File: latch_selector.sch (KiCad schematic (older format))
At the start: 15 parts, among them SW1 SW_Coded_Octal-8, U1 74HCT138, U2 74HCT151, U6 74HCT32

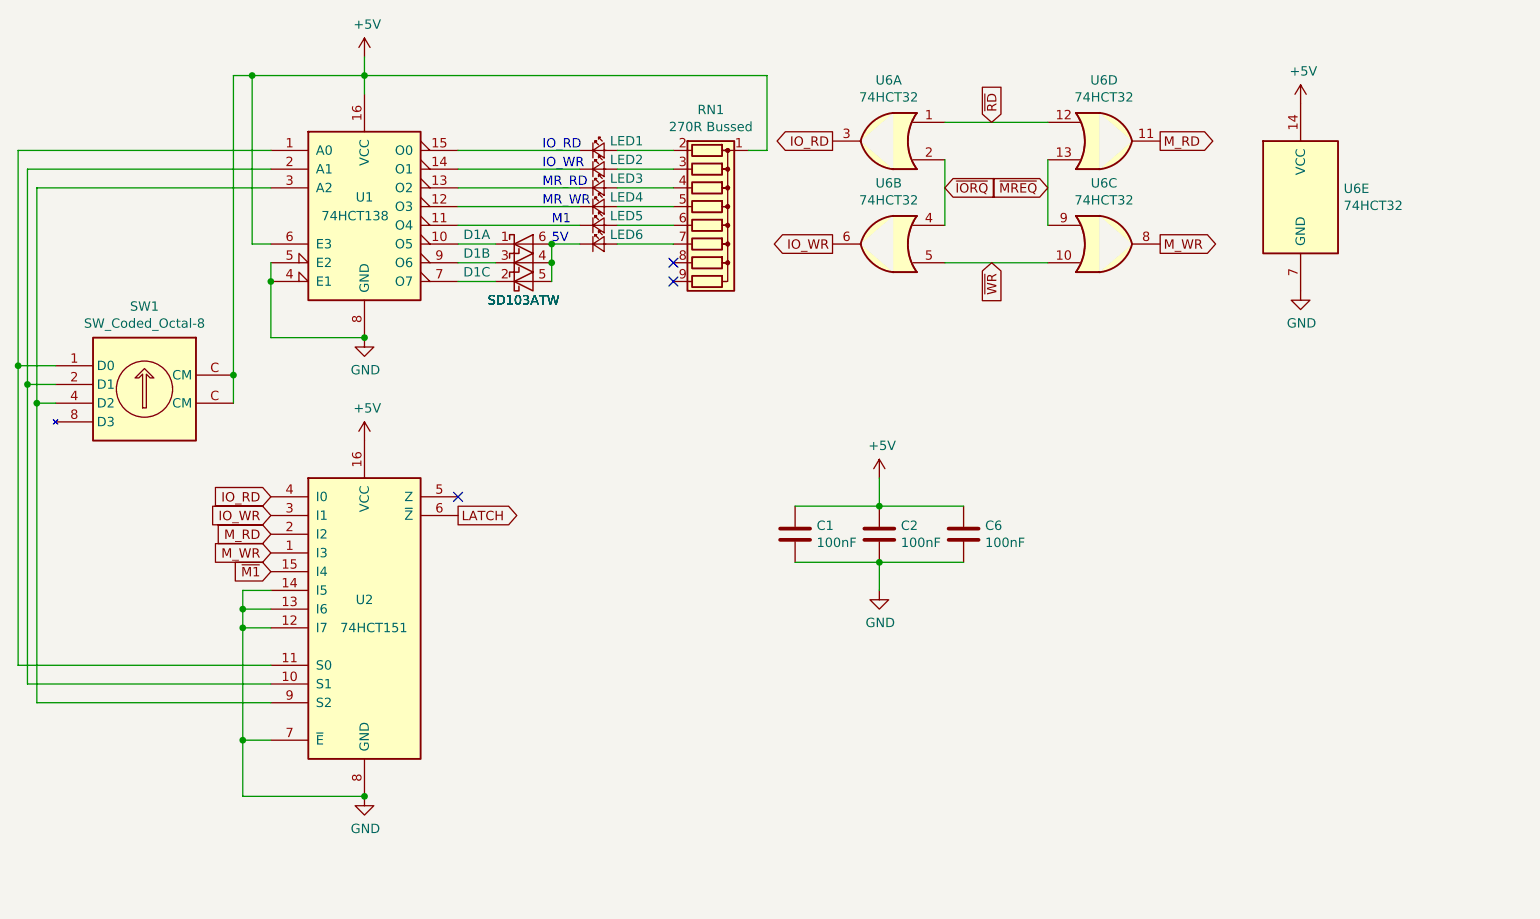
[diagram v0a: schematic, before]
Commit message: label updates
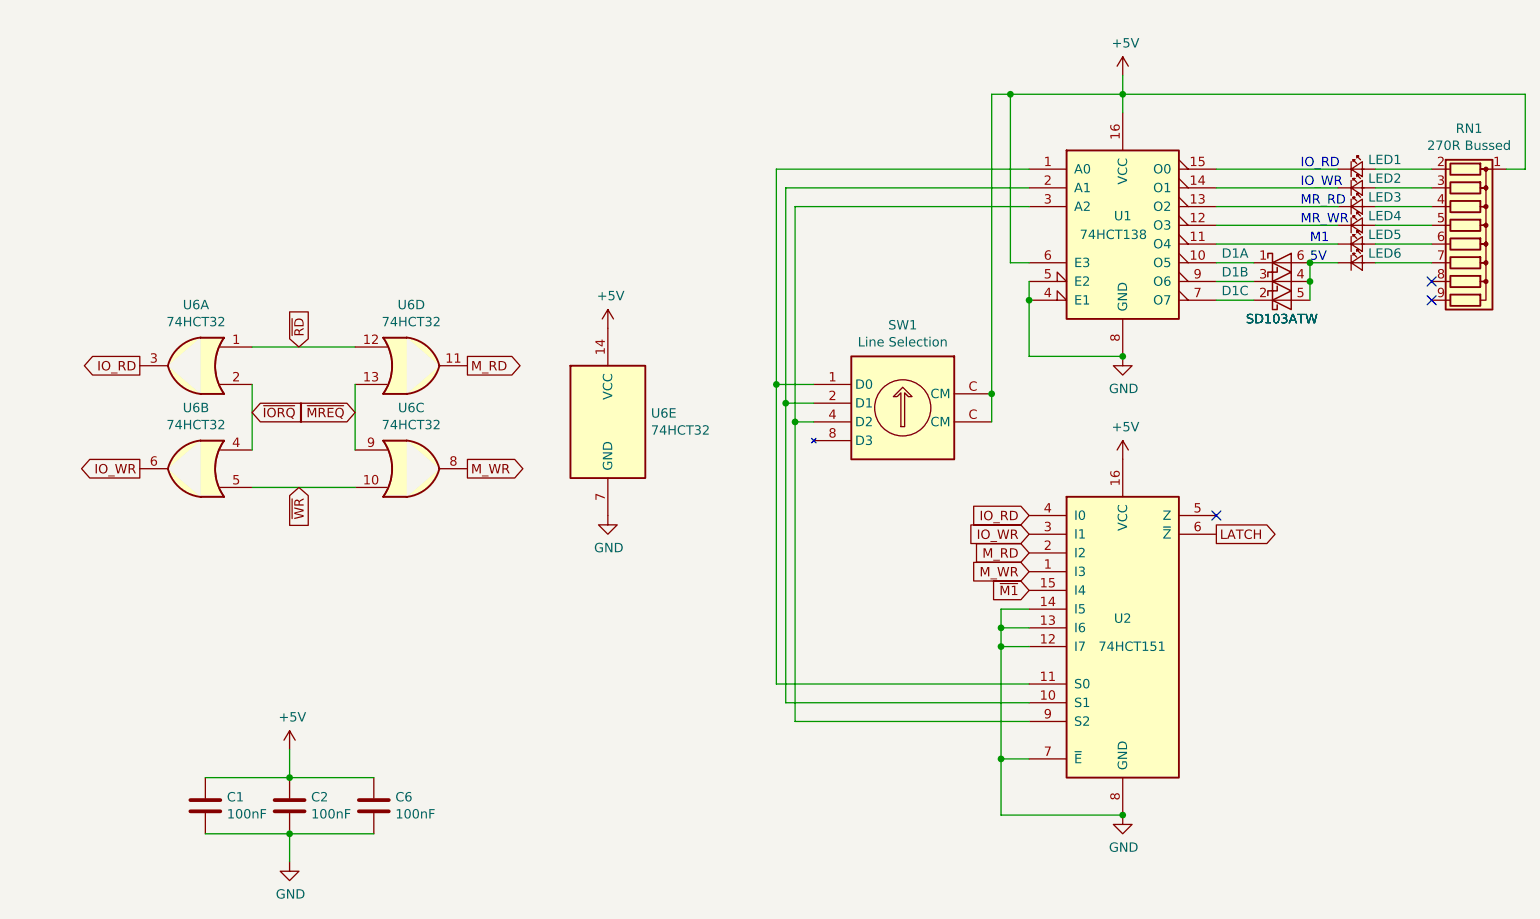
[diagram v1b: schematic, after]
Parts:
- SW1: value SW_Coded_Octal-8 -> Line Selection
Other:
- moved on the sheet: C1, C2, C6, D1A, D1B, D1C, LED1, LED2, LED3, LED4, LED5, LED6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
